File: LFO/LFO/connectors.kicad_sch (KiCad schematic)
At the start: 10 parts, among them J1 Conn_01x06, J13 Conn_02x05_Odd_Even, J3 Conn_01x06, J4 Conn_01x01, J5 Conn_01x01, J6 Conn_01x01, J7 Conn_01x01, J8 Conn_01x03

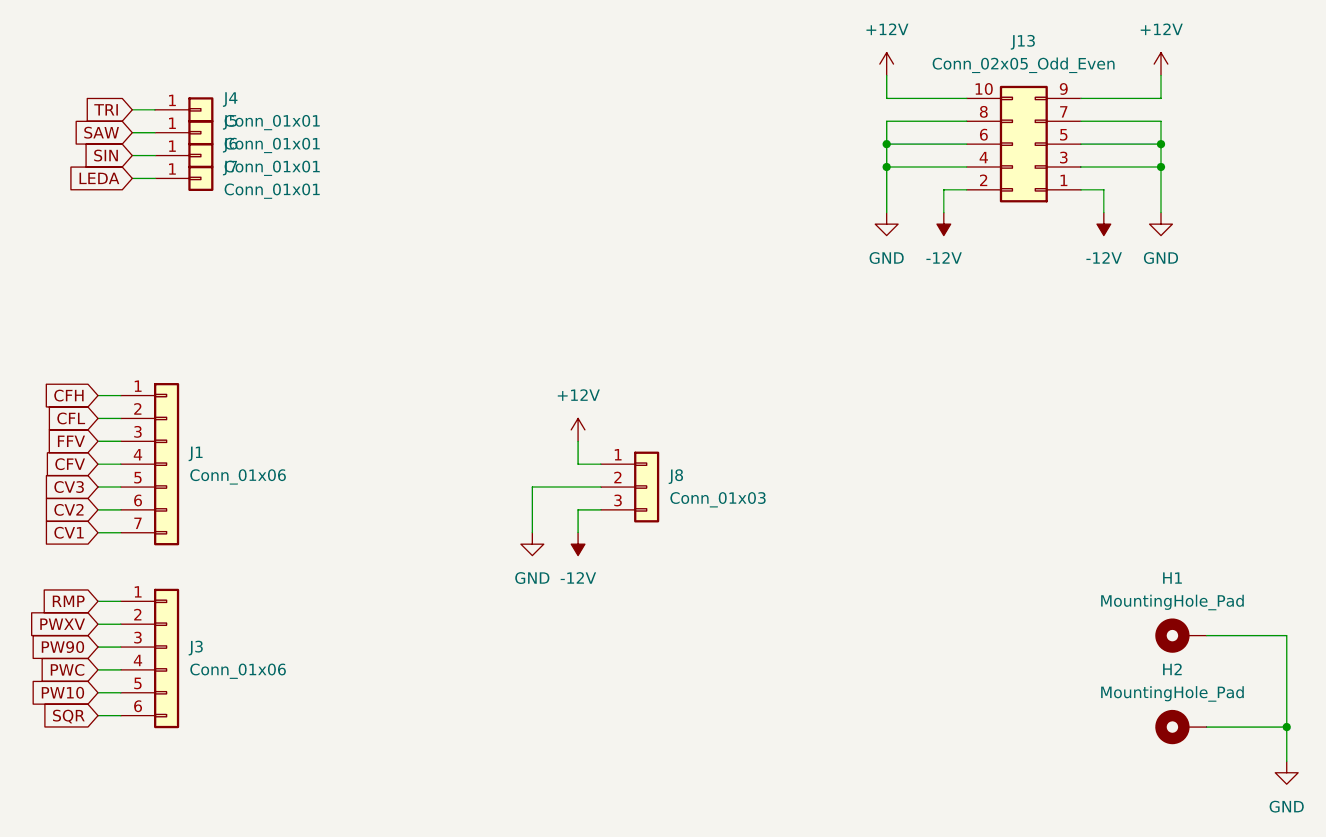
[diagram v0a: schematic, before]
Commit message: minor fixes after first build
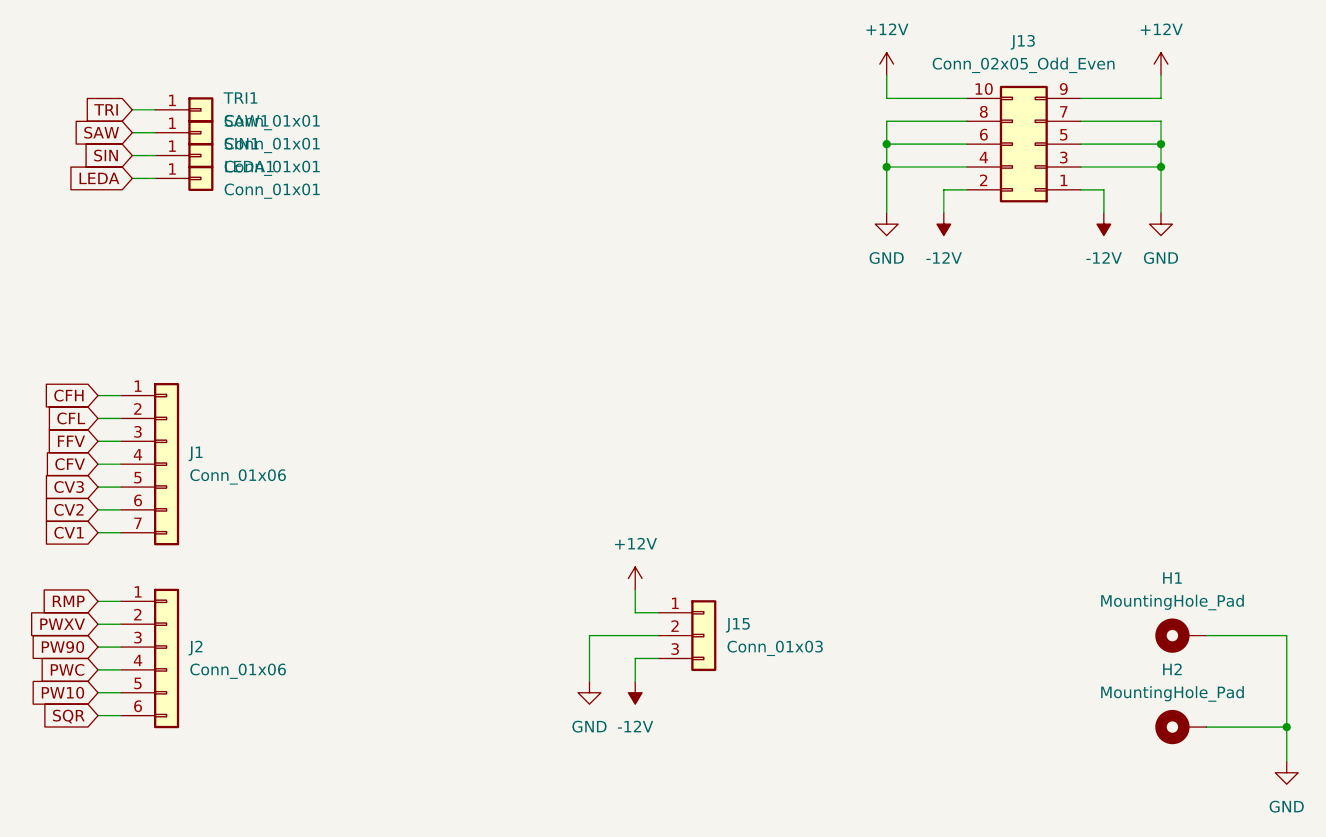
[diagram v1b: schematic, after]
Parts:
- removed J8: Conn_01x03, symbol Connector_Generic:Conn_01x03
- added J15: Conn_01x03, Connector_PinHeader_2.54mm:PinHeader_1x03_P2.54mm_Vertical, symbol Connector_Generic:Conn_01x03
- renumbered J3 to J2, J7 to LEDA1, J5 to SAW1, J6 to SIN1, J4 to TRI1
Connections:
- net +12V: now also J15.1 (Pin_1)
- net -12V: now also J15.3 (Pin_3)
- net GND: now also J15.2 (Pin_2)
